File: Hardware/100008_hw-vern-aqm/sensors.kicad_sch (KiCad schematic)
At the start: 5 parts

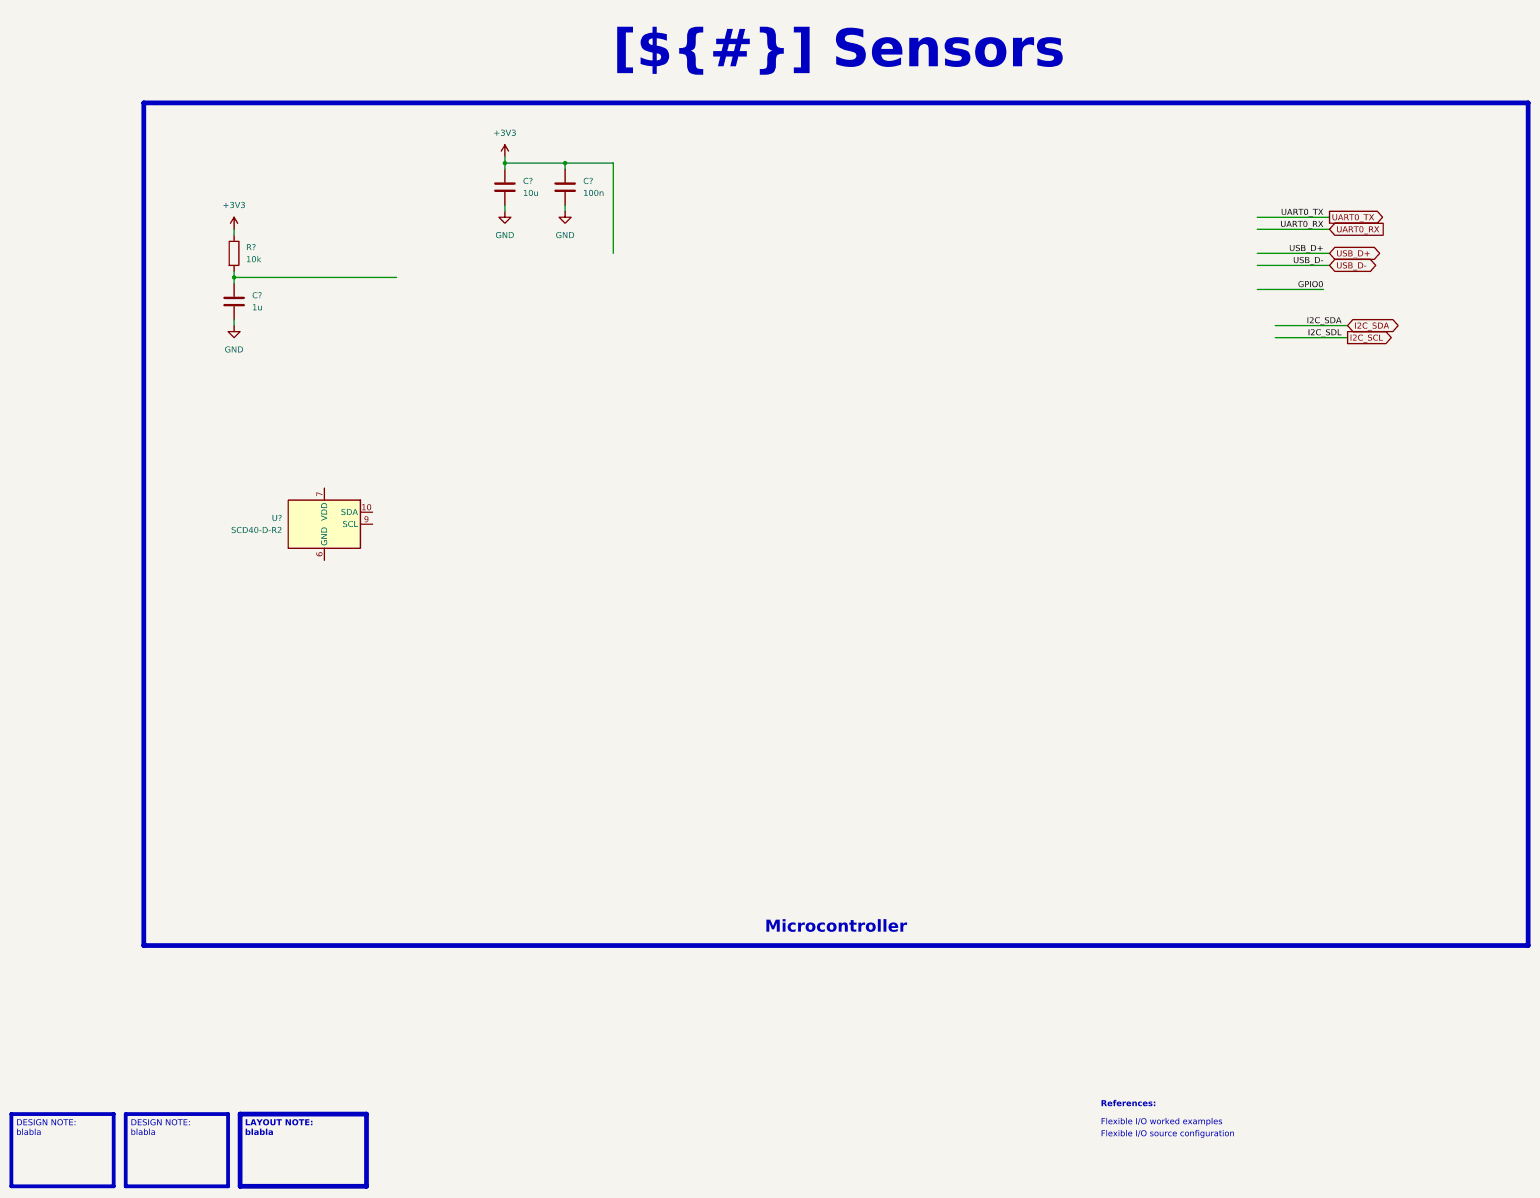
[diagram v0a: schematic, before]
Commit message: schematic work
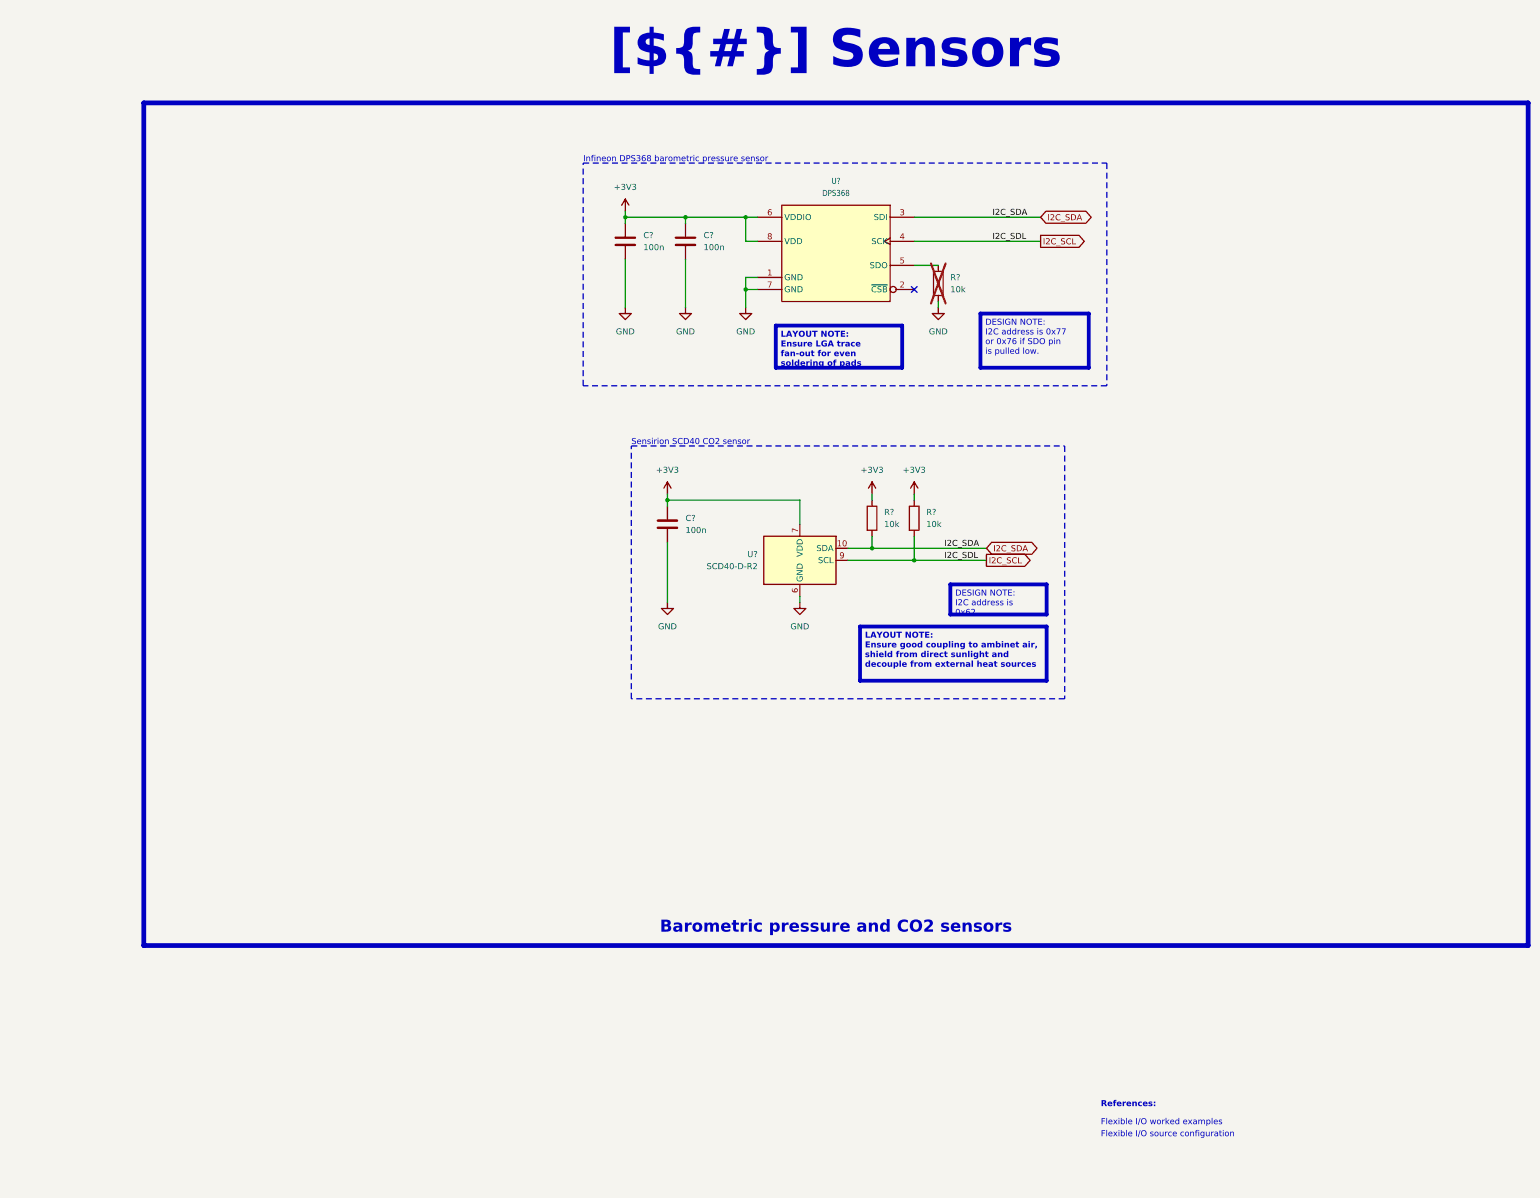
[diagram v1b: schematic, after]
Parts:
- removed C?: 10u, Capacitor_SMD:C_0805_2012Metric, symbol Device:C
- removed C?: 1u, Capacitor_SMD:C_0805_2012Metric, symbol Device:C
- removed C?: 100n, Capacitor_SMD:C_0603_1608Metric, symbol Device:C
- removed R?: 10k, Resistor_SMD:R_0603_1608Metric, symbol Device:R
- added C? (x3): 100n, Capacitor_SMD:C_0603_1608Metric, symbol Device:C
- added R? (x3): 10k, Resistor_SMD:R_0603_1608Metric, symbol Device:R
- added U?: DPS368, Components:LGA8S145X65P2X4_200X250X110-V, symbol ICs:DPS368
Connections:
- net +3V3: now also U?.19 (VDD), U?.7 (VDD), C?.1, C?.1, C?.1, R?.1, R?.1, U?.6 (VDDIO), U?.8 (VDD)
- net GND: now also U?.20 (GND), U?.21 (GND), U?.6 (GND), C?.2, C?.2, C?.2, R?.2, U?.1 (GND), U?.7 (GND)
- net I2C_SCL: now also U?.9 (SCL), R?.2, U?.4 (SCK)
- net I2C_SDA: now also U?.10 (SDA), R?.2, U?.3 (SDI)
- new net: R?.1, U?.5 (SDO)
- no-connect marks 0 -> 1
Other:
- note added: "Infineon DPS368 barometric pressure sensor"
- note added: "Sensirion SCD40 CO2 sensor"
- moved on the sheet: U?

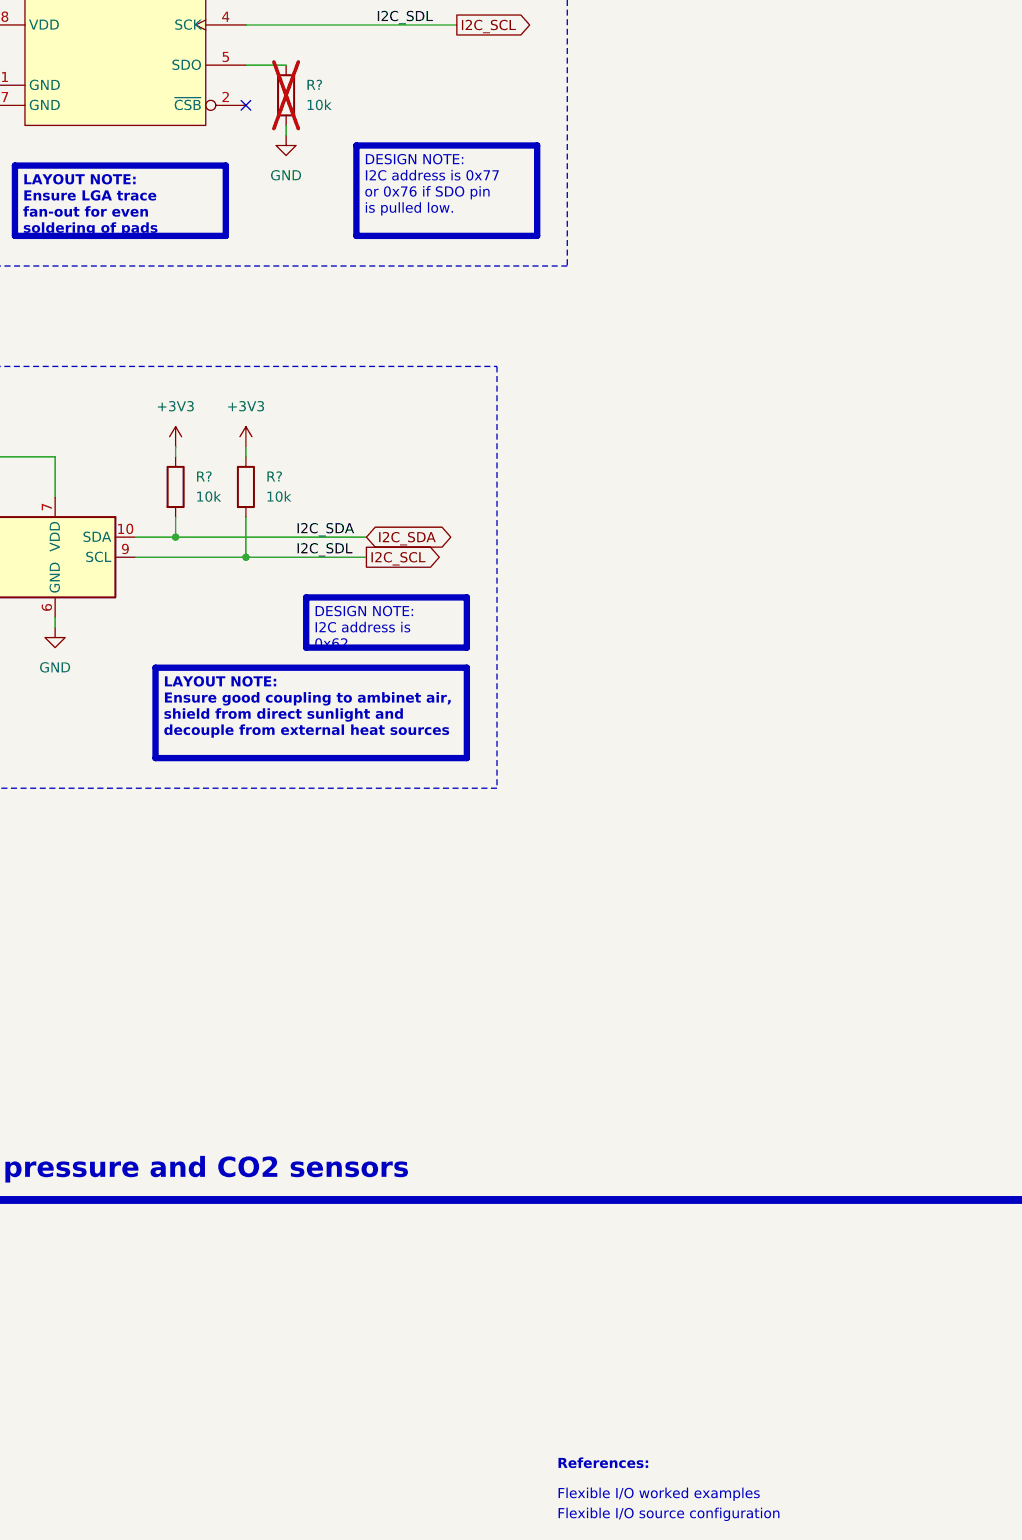
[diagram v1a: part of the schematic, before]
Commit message: schematic work
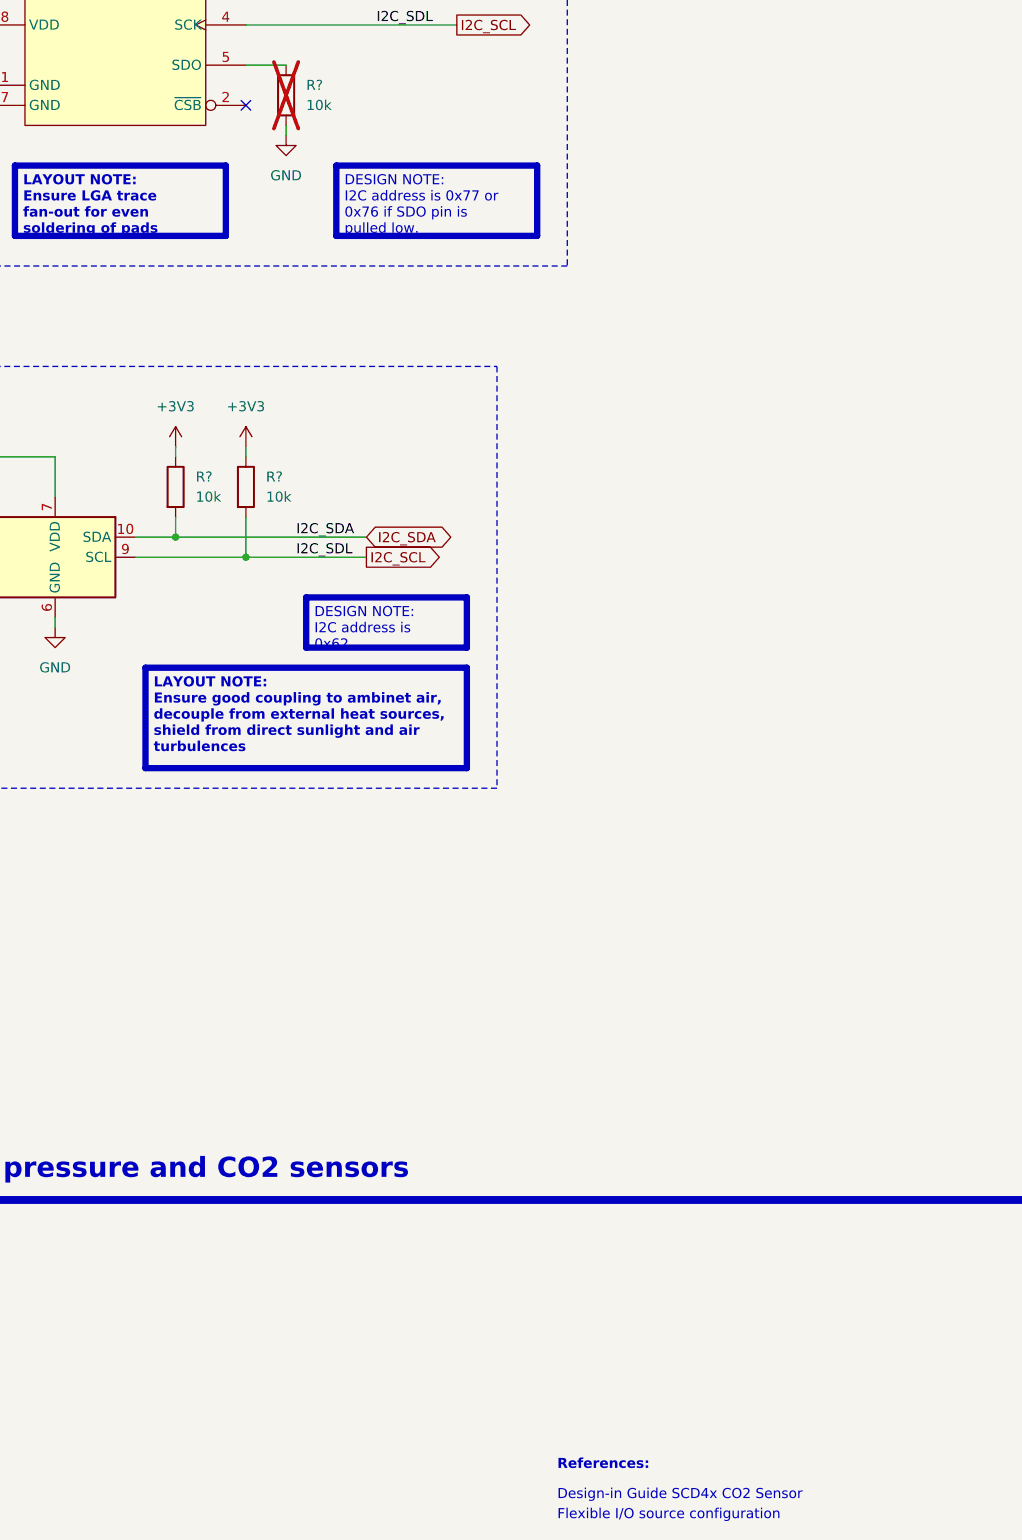
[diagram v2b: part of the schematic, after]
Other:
- note added: "Design-in Guide SCD4x CO2 Sensor"
- note removed: "Flexible I/O worked examples"
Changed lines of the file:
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@@
 		)
 	)
-	(text_box "LAYOUT NOTE:\nEnsure good coupling to ambinet air, shield from direct sunlight and decouple from external heat sources"
+	(text_box "LAYOUT NOTE:\nEnsure good coupling to ambinet air, decouple from external heat sources, shield from direct sunlight and air turbulences"
 		(exclude_from_sim no)
-		(at 214.63 148.59 0)
-		(size 39.37 11.43)
+		(at 213.36 148.59 0)
+		(size 40.64 12.7)
 		(stroke
 			(width 0.8)
@@
 	(text_box "DESIGN NOTE:\nI2C address is 0x77 or 0x76 if SDO pin is pulled low."
 		(exclude_from_sim no)
-		(at 240.03 82.55 0)
-		(size 22.86 11.43)
+		(at 237.49 85.09 0)
+		(size 25.4 8.89)
 		(stroke
 			(width 0.8)
@@
 		)
 	)
-	(text "Flexible I/O worked examples"
+	(text "Design-in Guide SCD4x CO2 Sensor"
 		(exclude_from_sim no)
 		(at 265.43 254 0)
@@
 			)
 			(justify left bottom)
-			(href "https://jpieper.com/2022/06/30/flexible-i-o-worked-examples/")
+			(href "https://sensirion.com/media/documents/0D0C9129/623B1183/Sensirion_CO2_Sensors_SCD4x_design-in_guide.pdf")
 		)
 	)
